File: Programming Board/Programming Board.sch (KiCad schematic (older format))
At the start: 4 parts, among them J2 SPOX-5, SW1 SW_Push, U1 DB20M

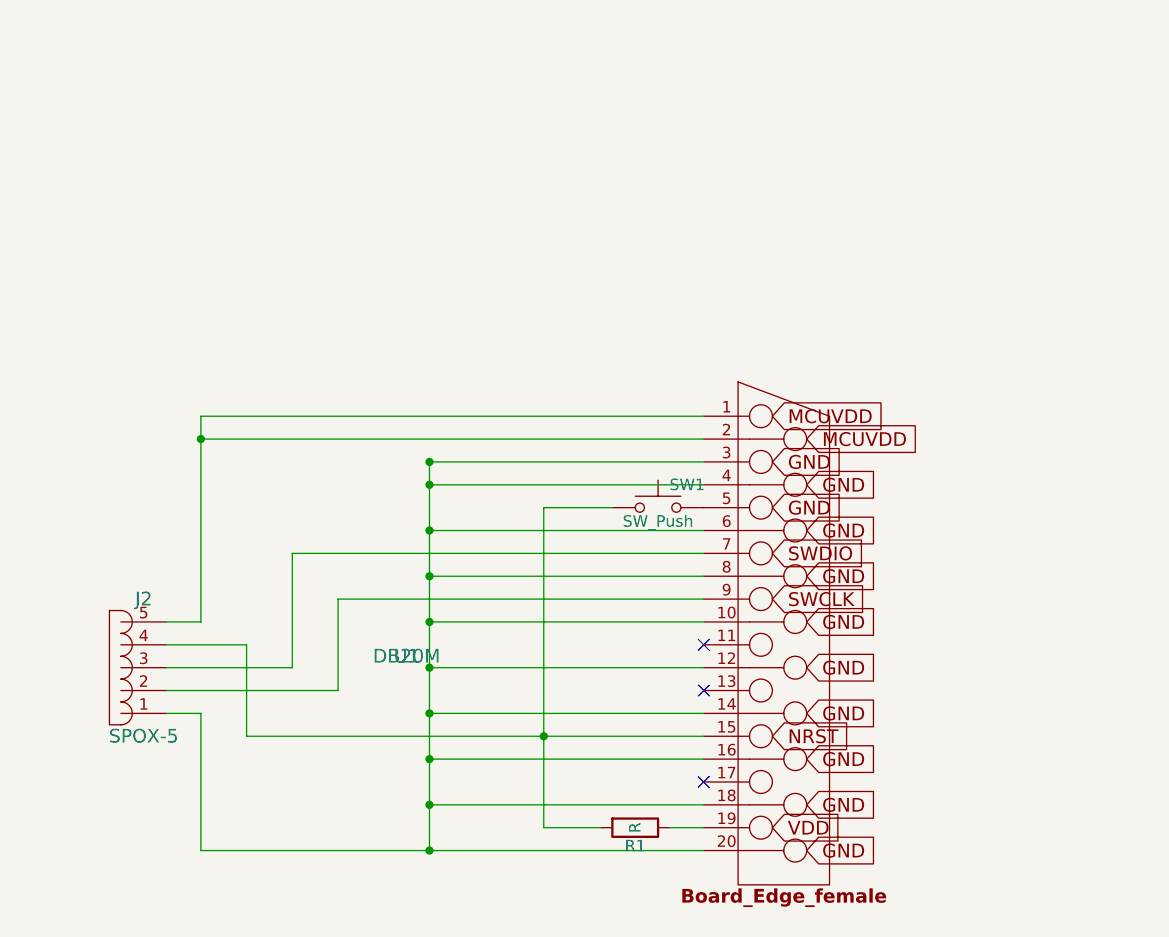
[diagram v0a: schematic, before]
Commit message: Add everything
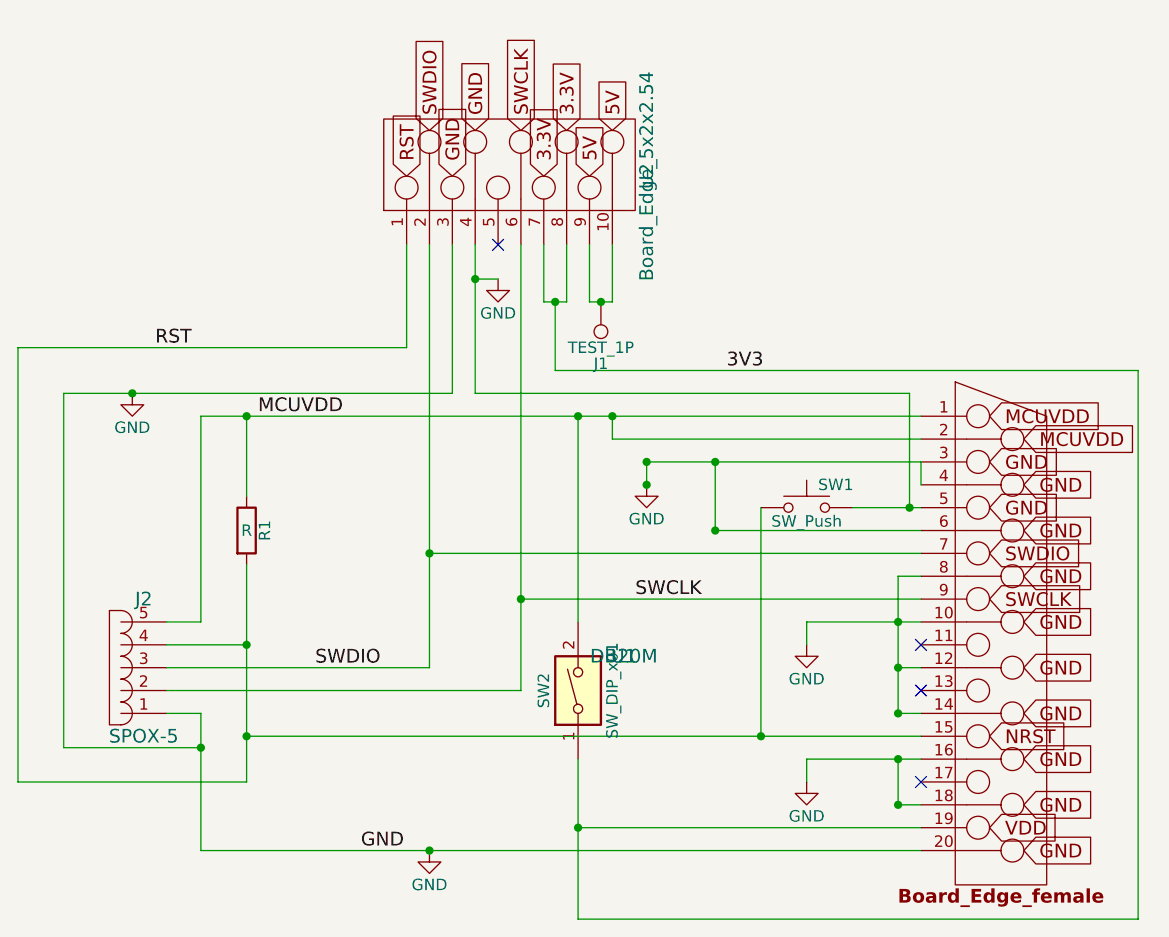
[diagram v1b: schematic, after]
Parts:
- added J1: TEST_1P, WARG KiCAD:Test_Point_5V, symbol TEST_1P
- added SW2: SW_DIP_x01, WARG KiCAD:Programming_Board_Switch, symbol SW_DIP_x01
- added U2: Board_Edge_5x2x2.54, WARG KiCAD:Board_Edge_Female2x5x2.54, symbol Board_Edge_5x2x2.54
- J2: footprint (none) -> Connectors_Molex:Molex_SPOX-5267_22-03-5055_05x2.54mm_Straight
- SW1: footprint (none) -> WARG KiCAD:Programmer_ResetButton
- U1: footprint WARG-kicad:Board_Edge_female -> WARG KiCAD:Board_Edge_10x2x2.54
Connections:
- net GND: now also J2.1, SW1.2, U1.10, U1.12, U1.14, U1.16, U1.18, U1.20, U1.3, U1.4, U1.5, U1.6, U1.8, U2.3, U2.4
- net MCUVDD: now also J2.5, R1.1, U1.1, U1.2, SW2.2
- net SWCLK: now also J2.2, U1.9, U2.6
- net SWDIO: now also J2.3, U1.7, U2.2
- net RST: now reaches J2.4, R1.2, SW1.1, U1.15
- net RST: now also U2.1
- net 3V3: now reaches U1.19
- net 3V3: now also SW2.1, U2.7, U2.8; no longer R1.1
- new net: J1.1, U2.10, U2.9
- no-connect marks 3 -> 4
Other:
- moved on the sheet: R1, SW1, U1
